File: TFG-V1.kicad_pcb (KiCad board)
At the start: 2 copper layers, 55 x 90 mm, 69 parts, among them CN1 1n, CN2 1n, CN3 1n, CN4 1n, CN5 1n, J1 Input, U1 AMS1117-3.3, U10 TPS72325, U11 TPD4E1U06, U12 CRE1S0505SC, U14 ESP32-C3-DevKitC-02, U15 ADuM3151, U2 TPD4E1U06, U3 ADS1298PAG, U4 TPD4E1U06, U5 LM2664, U6 MIC5504-2.5YM5, U7 TPD4E1U06, U8 TPD4E1U06, U9 TPD4E1U06

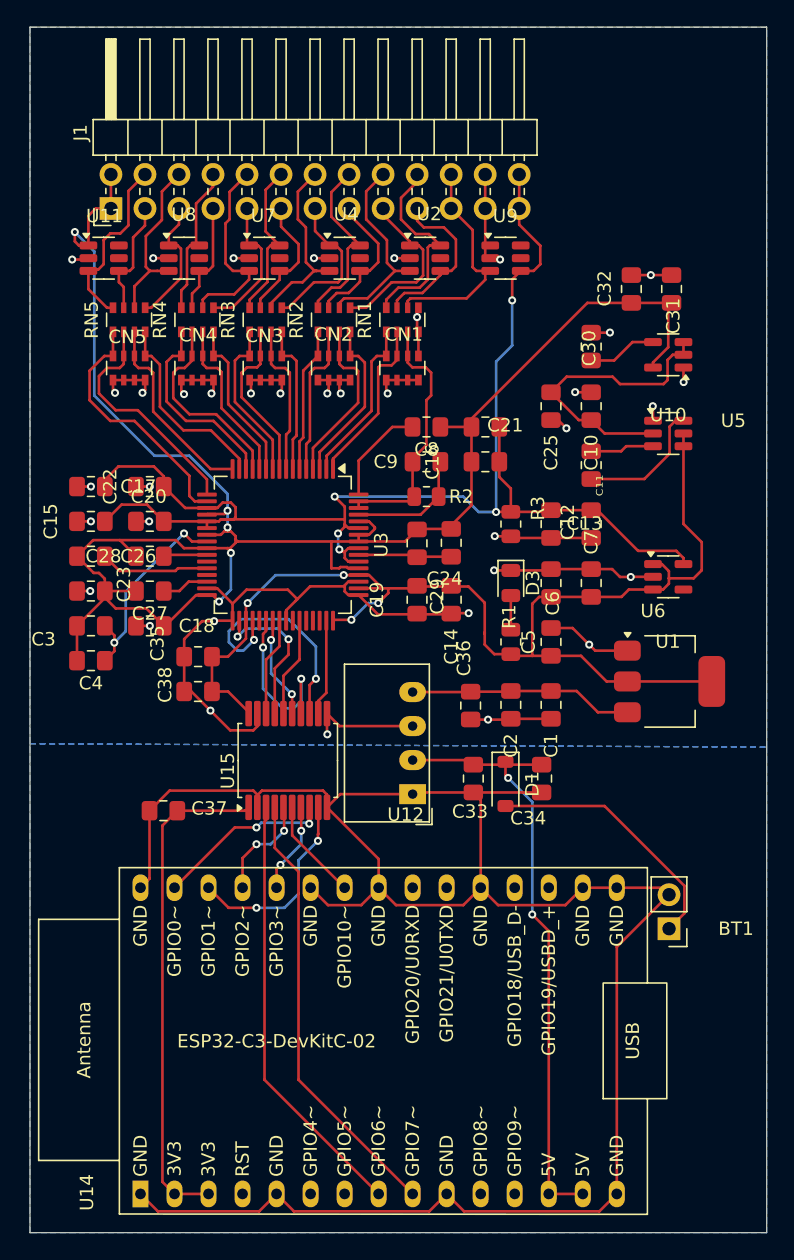
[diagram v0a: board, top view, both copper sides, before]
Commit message: diseño final
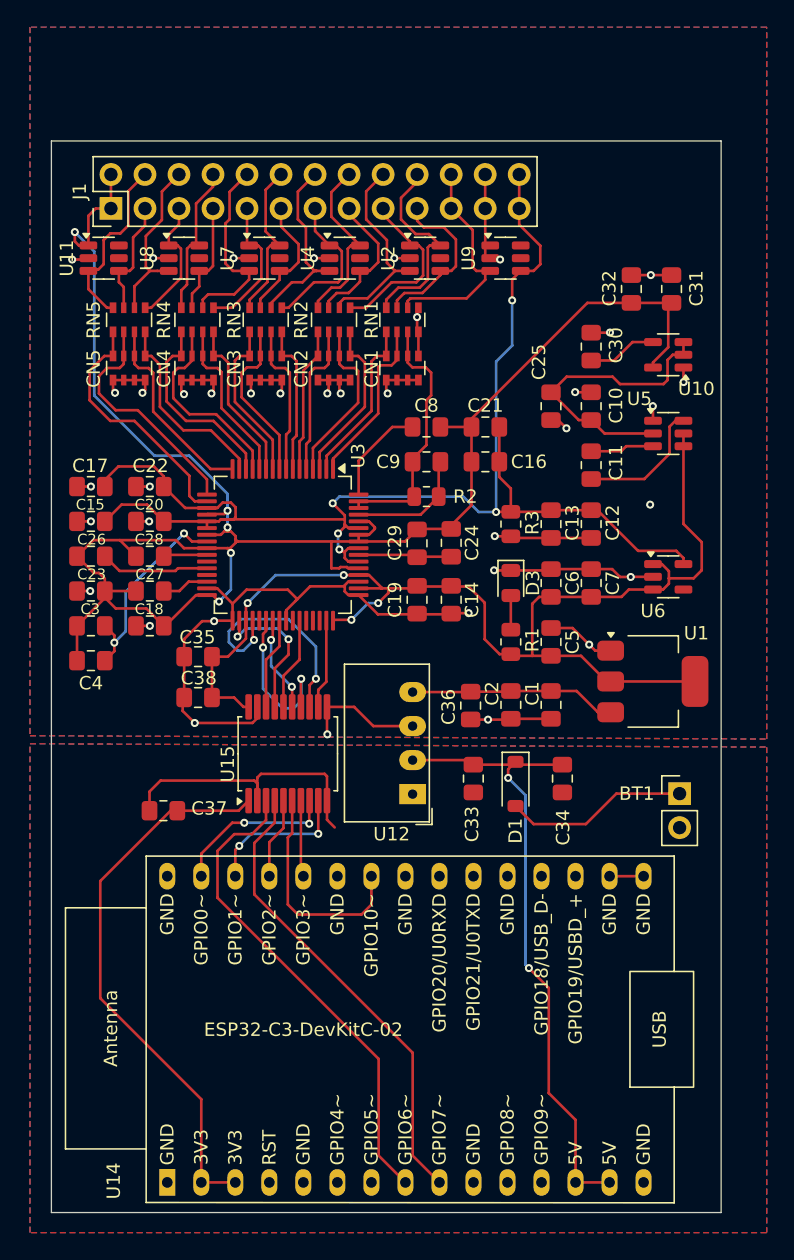
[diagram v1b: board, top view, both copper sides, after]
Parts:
- J1: footprint Connector_PinHeader_2.54mm:PinHeader_2x13_P2.54mm_Horizontal -> Connector_PinHeader_2.54mm:PinHeader_2x13_P2.54mm_Vertical
- moved BT1 10.1 mm to (151.0, 89.5), turned to 0 degrees
- moved U14 2.18 mm to (112.8, 118.5)
- moved C34 1.55 mm to (142.2, 88.3)
- moved U1 1.25 mm to (149.0, 81.1)
- moved D1 0.75 mm to (138.8, 88.8)
- moved U15 0.50 mm to (121.8, 86.5)
- moved C38 0.45 mm to (115.0, 82.3)
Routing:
- net GND: track 147.5 -> 24.9 mm
- net /FE_CS: track 7.62 -> 16.9 mm
- net /BAT_IN: track 19.5 -> 13.8 mm
- net 3V3: track 37.4 -> 41.7 mm
- net /SPI1_SCLK: track 32.4 -> 36.6 mm
- net /FE_DRDY: track 14.8 -> 11.1 mm
- net /SPI1_MISO: track 7.93 -> 6.08 mm, vias 2 -> 0
- net /SPI1_MOSI: track 33.1 -> 34.9 mm
- net +5V: track 46.1 -> 47.8 mm
- net VDD: track 90.3 -> 88.8 mm
- net /5V_ISO: track 16.7 -> 15.5 mm
- net /FE_START: track 6.77 -> 5.72 mm, vias 2 -> 0
- net /FE_RESET: track 13.3 -> 12.5 mm
- net /SPI1_SCLK_ISO: track 7.35 -> 6.85 mm
- net /SPI1_MOSI_ISO: track 11.6 -> 11.1 mm
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- added copper zone on F.Cu, net GND
- added copper zone on F.Cu, net GNDD
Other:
- board size 55 x 90 mm -> 50 x 80 mm
